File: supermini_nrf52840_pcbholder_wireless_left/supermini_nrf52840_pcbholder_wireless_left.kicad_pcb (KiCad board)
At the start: 2 copper layers, 34.3 x 38.3 mm, 9 parts, among them J10 Conn_01x08_Pin, J5 Conn_01x02_Pin, J7 Conn_01x04_Pin, J9 Conn_01x08_Pin, SW2 SW_SPST, SW3 SW_SPDT, U5 nice_nano

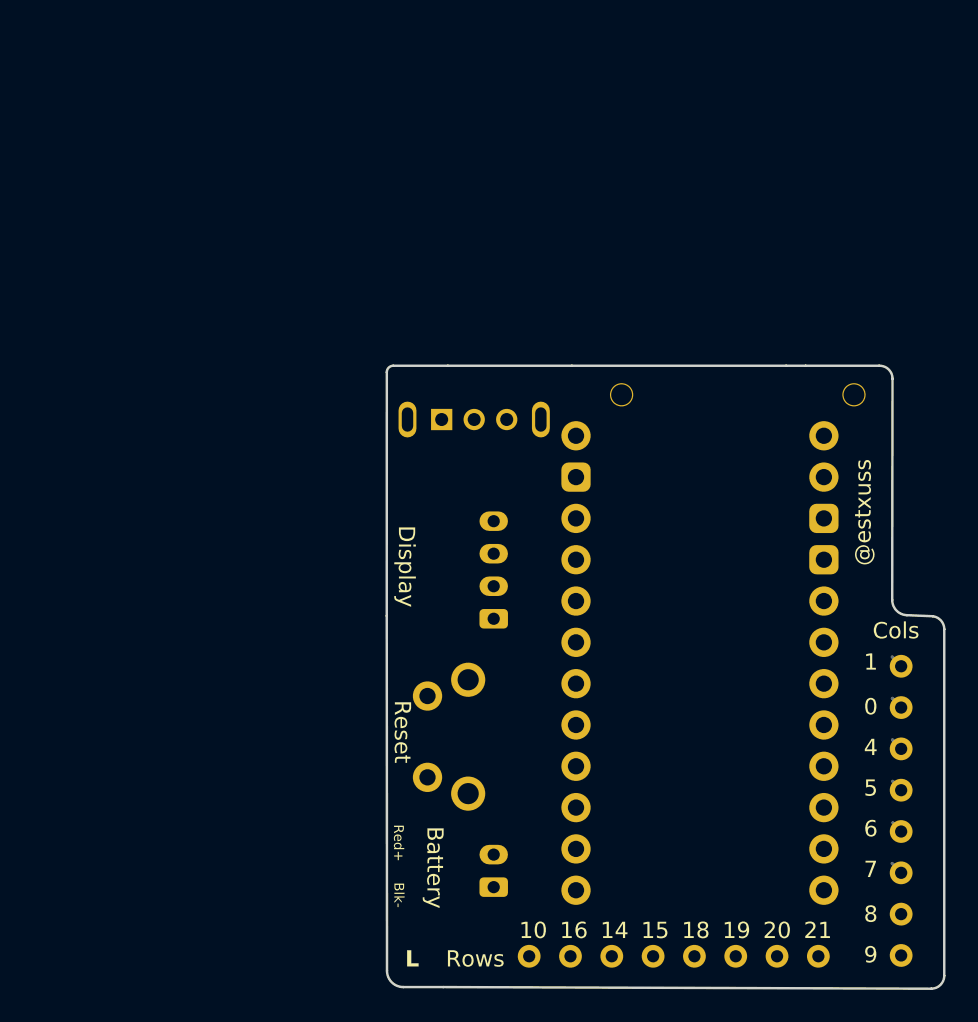
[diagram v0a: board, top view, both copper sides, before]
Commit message: create left side and tweaks
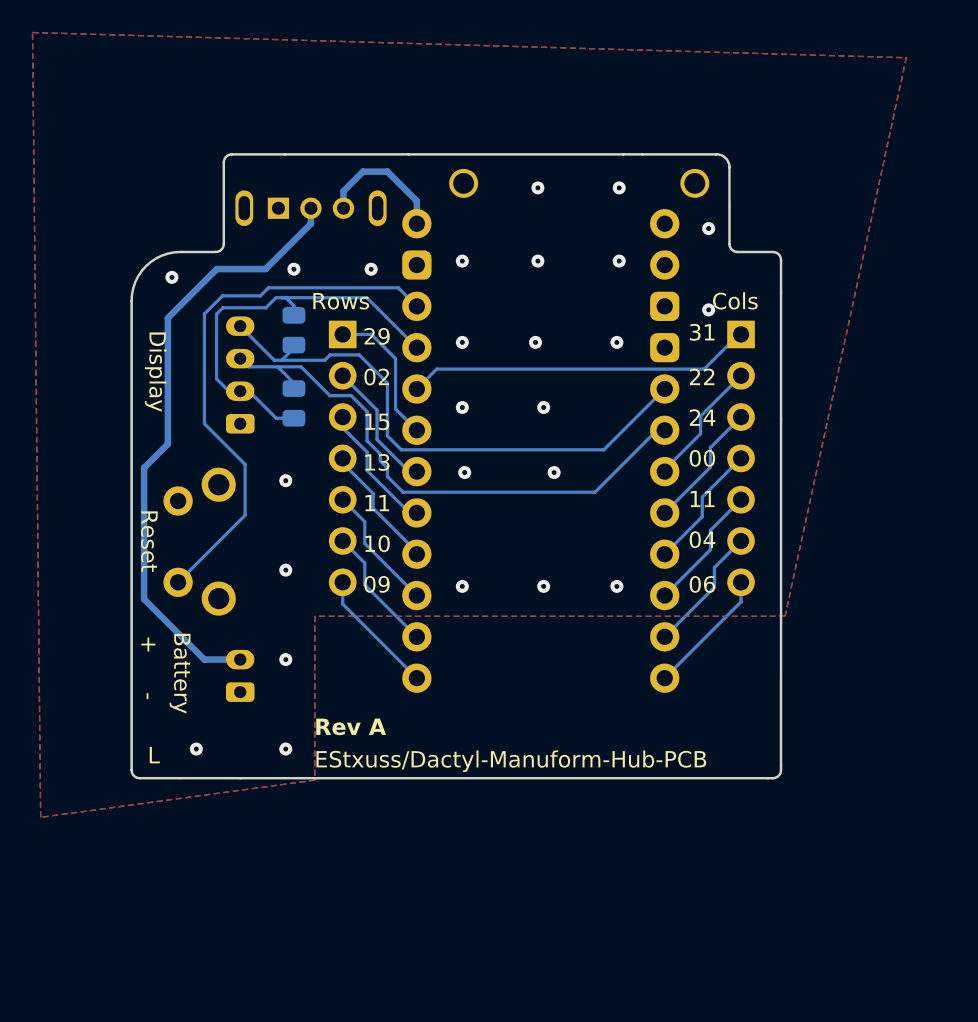
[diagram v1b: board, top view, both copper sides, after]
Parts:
- removed H3, H4: MountingHole, #footprint:M1.4_tapping_Hole_rev2
- removed J10, J9: Conn_01x08_Pin, #footprint:PinHeader_1x08_P2.54mm_Vertical_rev2
- removed J5: Conn_01x02_Pin, Connector_JST:JST_PH_S2B-PH-K_1x02_P2.00mm_Horizontal
- removed J7: Conn_01x04_Pin, Connector_JST:JST_PH_S4B-PH-K_1x04_P2.00mm_Horizontal
- removed SW3: SW_SPDT, SLW_864574_5A_RA_N_D:SW_SLW-864574-5A-RA-N-D
- removed U5: nice_nano, PCM_marbastlib-xp-promicroish:SuperMini_nRF52840_H_USBup
- added H1: MountingHole, mounting-hole:M1.4_tapping_Hole_JLC, F.Cu at (137.6, 63.7)
- added H2: MountingHole, mounting-hole:M1.4_tapping_Hole_JLC, F.Cu at (123.4, 63.7)
- added J1: Conn_01x02, Connector_JST:JST_PH_S2B-PH-K_1x02_P2.00mm_Horizontal, B.Cu at (109.7, 95.0)
- added J2: Conn_01x04, Connector_JST:JST_PH_S4B-PH-K_1x04_P2.00mm_Horizontal, B.Cu at (109.7, 78.5)
- added J3: Conn_01x07, Connector_PinHeader_2.54mm:PinHeader_1x07_P2.54mm_Vertical, B.Cu at (140.5, 73.0)
- added J4: Conn_01x07, Connector_PinHeader_2.54mm:PinHeader_1x07_P2.54mm_Vertical, B.Cu at (116.0, 73.0)
- added R1: 4.7k, Resistor_SMD:R_0805_2012Metric, B.Cu at (113.0, 77.2)
- added R2: 4.7k, Resistor_SMD:R_0805_2012Metric, B.Cu at (113.0, 72.8)
- added SW1: SW_SPDT, SLW_864574_5A_RA_N_D:SW_SLW-864574-5A-RA-N-D, B.Cu at (114.0, 65.2)
- added U1: nice_nano, PCM_marbastlib-xp-promicroish:SuperMini_nRF52840_H_USBup, B.Cu at (128.2, 80.2)
- moved SW2 19.5 mm to (107.1, 85.8)
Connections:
- SW2 pad 1: (no net) -> Net-(SW2-A)
- SW2 pad 2: (no net) -> GND
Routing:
- net /BATT_SW_POS: track 0.00 -> 37.5 mm
- net /OLED_SCL: track 0.00 -> 34.4 mm
- net /OLED_SDA: track 0.00 -> 34.2 mm
- net Net-(SW2-A): track 0.00 -> 33.4 mm
- net VCC: track 0.00 -> 25.3 mm
- net COL1: track 0.00 -> 21.3 mm
- net /ROW1: track 0.00 -> 8.81 mm
- net /BATT_POS: track 0.00 -> 8.20 mm
- net /ROW2: track 0.00 -> 8.06 mm
- net /ROW3: track 0.00 -> 8.04 mm
- net /COL7: track 0.00 -> 8.00 mm
- net /ROW5: track 0.00 -> 7.91 mm
- net /ROW4: track 0.00 -> 7.84 mm
- net /COL6: track 0.00 -> 7.84 mm
- net /COL5: track 0.00 -> 7.84 mm
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- added copper zone on B.Cu, net GND
- added copper zone on F.Cu, net GND
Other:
- board size 34.3 x 38.3 mm -> 39.9 x 38.4 mm
- board text added: "+"
- board text added: "-"
- board text added: "00"
- board text added: "02"
- board text added: "04"
- board text added: "06"
- board text added: "09"
- board text added: "11"
- board text added: "13"
- board text added: "22"
- board text added: "24"
- board text added: "29"
- board text added: "31"
- board text added: "EStxuss/Dactyl-Manuform-Hub-PCB"
- board text added: "Rev A"
- board text removed: "0"
- board text removed: "1"
- board text removed: "14"
- board text removed: "16"
- board text removed: "18"
- board text removed: "19"
- board text removed: "20"
- board text removed: "21"
- board text removed: "4"
- board text removed: "5"
- board text removed: "6"
- board text removed: "7"
- board text removed: "8"
- board text removed: "9"
- board text removed: "@estxuss"
- board text removed: "Blk-"
- board text removed: "Red+"
